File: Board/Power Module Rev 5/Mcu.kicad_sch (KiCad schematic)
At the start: 4 parts, among them J4 Conn_ARM_SWD_TagConnect_TC203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, J4 USB_C_Receptacle_USB2.0, U1 STM32G491CCUx, U6 MB85RS64

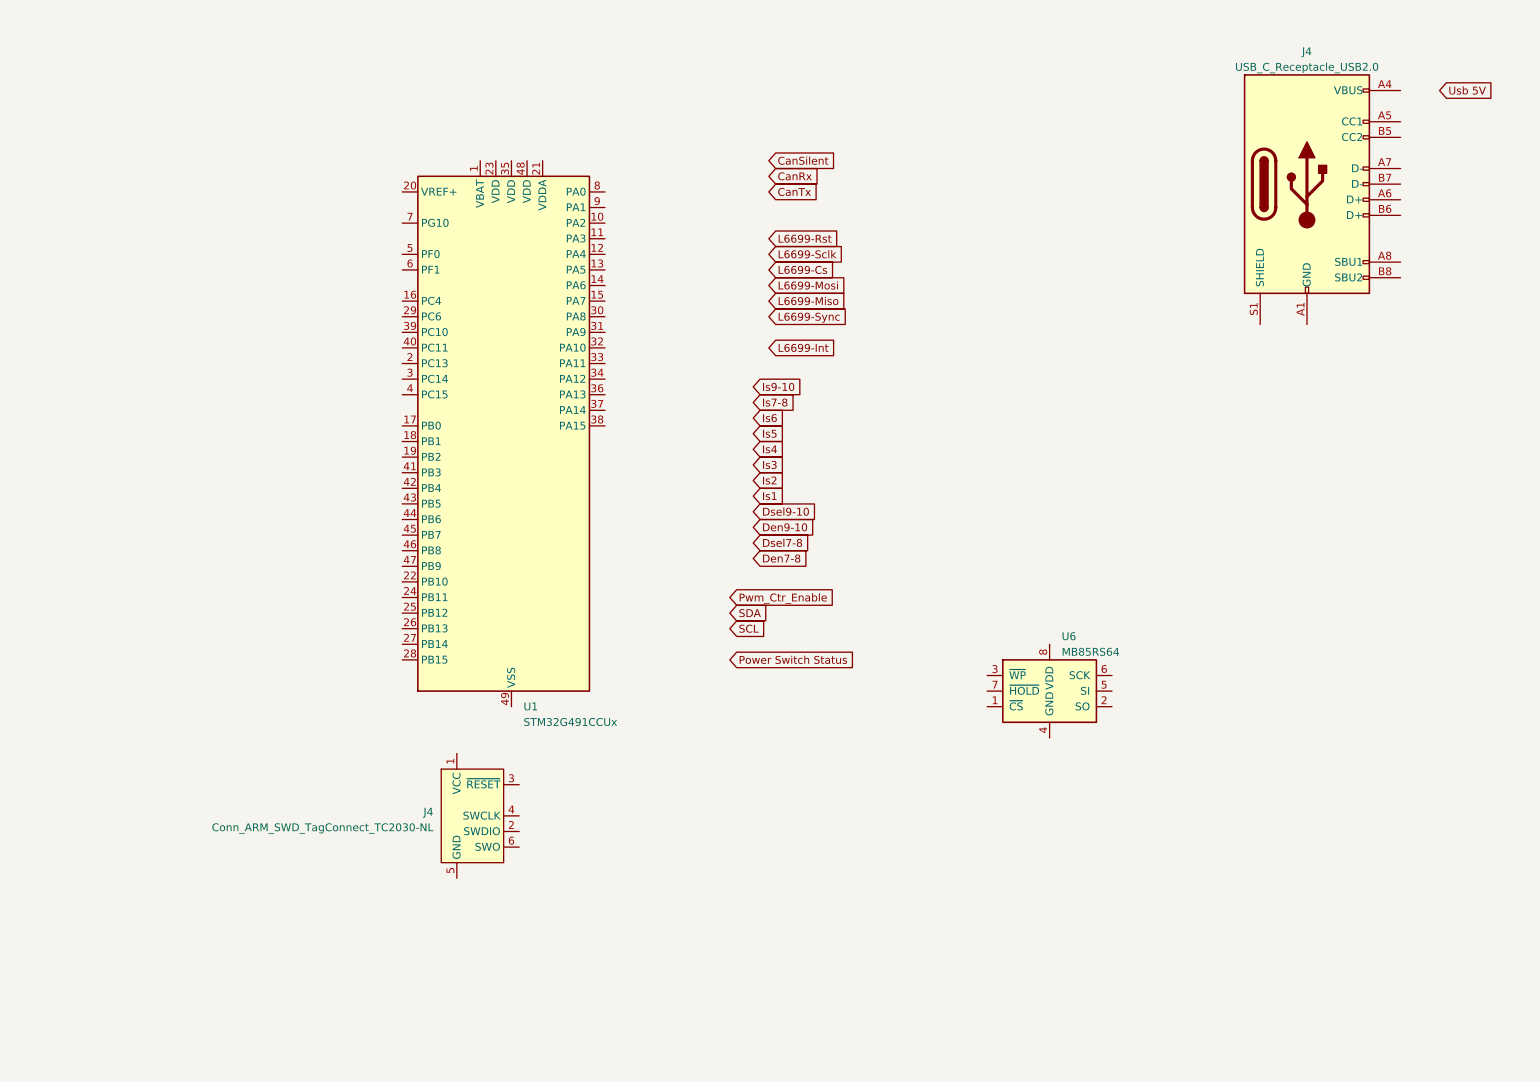
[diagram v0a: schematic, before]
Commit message: Board Update
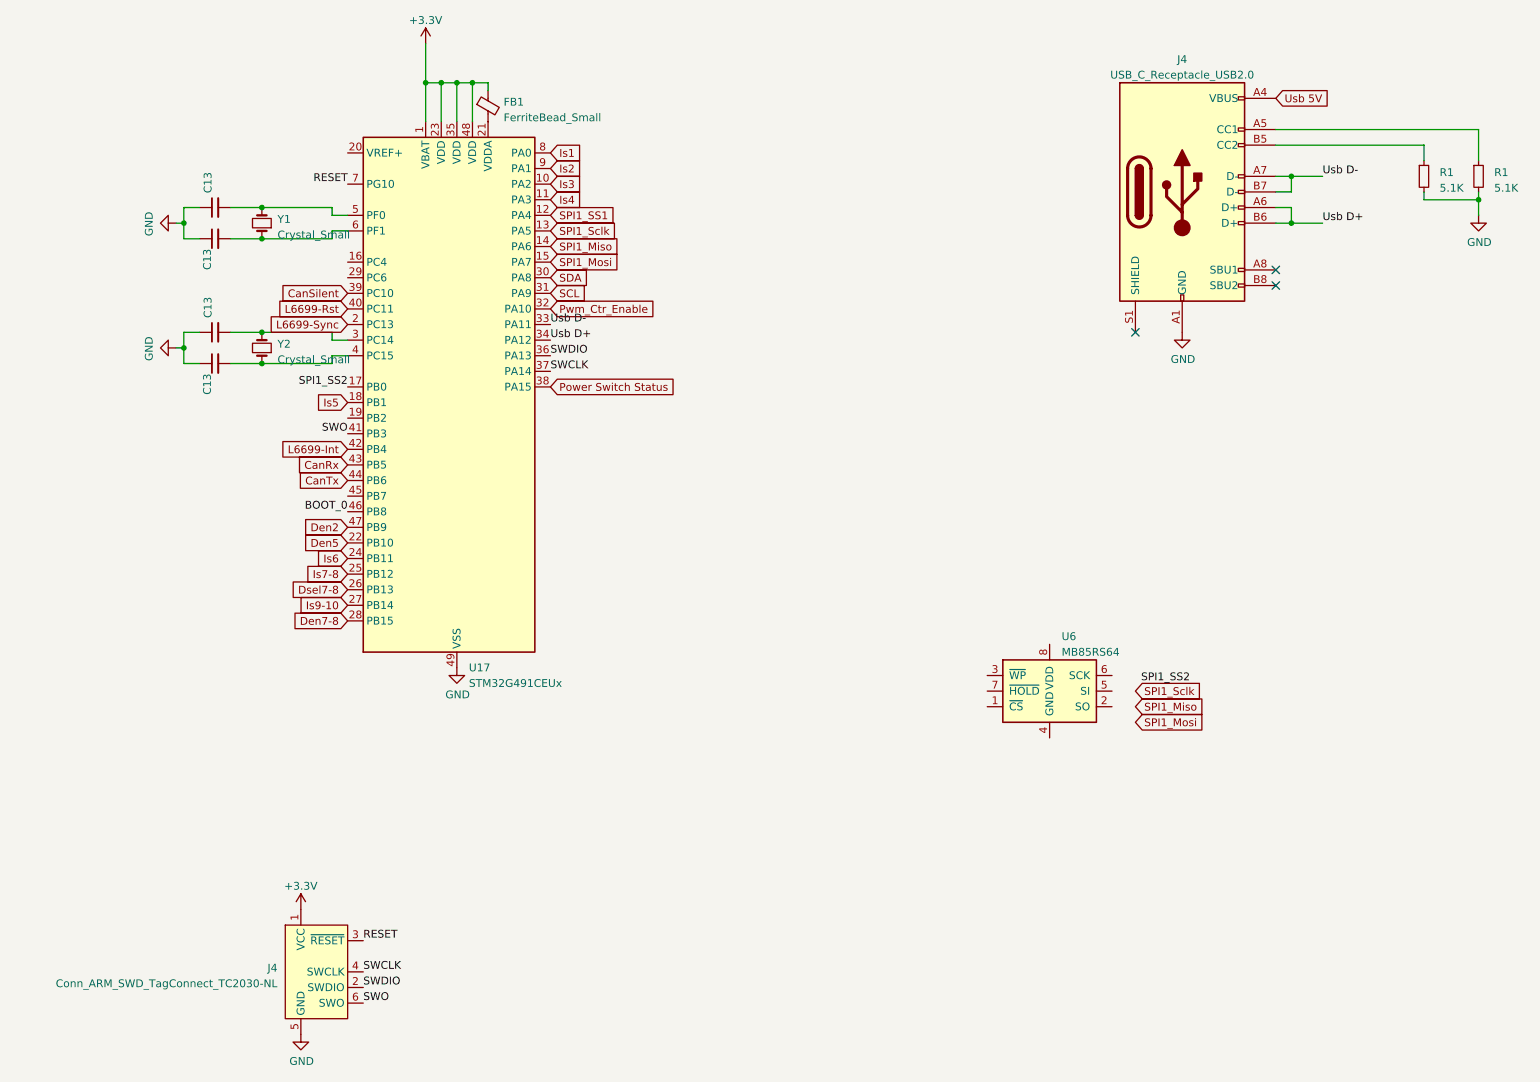
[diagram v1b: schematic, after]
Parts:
- removed U1: STM32G491CCUx, Package_DFN_QFN:QFN-48-1EP_7x7mm_P0.5mm_EP5.6x5.6mm, symbol MCU_ST_STM32G4:STM32G491CCUx
- added C13 (x4): ~, Capacitor_SMD:C_0603_1608Metric_Pad1.08x0.95mm_HandSolder, symbol Device:C_Small
- added FB1: FerriteBead_Small, Resistor_SMD:R_0603_1608Metric_Pad0.98x0.95mm_HandSolder, symbol Device:FerriteBead_Small
- added R1 (x2): 5.1K, Resistor_SMD:R_0603_1608Metric_Pad0.98x0.95mm_HandSolder, symbol Device:R_Small
- added U17: STM32G491CEUx, Package_DFN_QFN:QFN-48-1EP_7x7mm_P0.5mm_EP5.6x5.6mm, symbol MCU_ST_STM32G4:STM32G491CEUx
- added Y1, Y2: Crystal_Small, Crystal:Crystal_SMD_5032-2Pin_5.0x3.2mm, symbol Device:Crystal_Small
- J4: footprint (none) -> Connector_USB:USB_C_Receptacle_JAE_DX07S016JA1R1500
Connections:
- net CanRx: now also U17.43 (PB5)
- net CanSilent: now also U17.39 (PC10)
- net CanTx: now also U17.44 (PB6)
- net Den7-8: now also U17.28 (PB15)
- net Dsel7-8: now also U17.26 (PB13)
- net Is1: now also U17.8 (PA0)
- net Is2: now also U17.9 (PA1)
- net Is3: now also U17.10 (PA2)
- net Is4: now also U17.11 (PA3)
- net Is5: now also U17.18 (PB1)
- net Is6: now also U17.24 (PB11)
- net Is7-8: now also U17.25 (PB12)
- net Is9-10: now also U17.27 (PB14)
- net L6699-Int: now also U17.42 (PB4)
- net L6699-Rst: now also U17.40 (PC11)
- net L6699-Sync: now also U17.2 (PC13)
- net Power Switch Status: now also U17.38 (PA15)
- net Pwm_Ctr_Enable: now also U17.32 (PA10)
- net SCL: now also U17.31 (PA9)
- net SDA: now also U17.30 (PA8)
- net Usb 5V: now also J4.A4 (VBUS), J4.A9 (VBUS), J4.B4 (VBUS), J4.B9 (VBUS)
- net GND: now reaches J4.A1 (GND), J4.A12 (GND), J4.B1 (GND), J4.B12 (GND)
- net GND: now also J4.5 (GND), C13.1, C13.1, C13.1, C13.1, R1.2, R1.2, U17.49 (VSS)
- net at J4.A5 (CC1): now also R1.1
- net Usb D+: now reaches J4.A6 (D+)
- net Usb D+: now also J4.B6 (D+), U17.34 (PA12)
- net Usb D-: now reaches J4.A7 (D-)
- net Usb D-: now also J4.B7 (D-), U17.33 (PA11)
- net at J4.B5 (CC2): now also R1.1
- net +3.3V: now reaches J4.1 (VCC)
- net +3.3V: now also FB1.1, U17.1 (VBAT), U17.23 (VDD), U17.35 (VDD), U17.48 (VDD)
- net SWDIO: now reaches J4.2 (SWDIO)
- net SWDIO: now also U17.36 (PA13)
- net RESET: now reaches J4.3 (~{RESET})
- net RESET: now also U17.7 (PG10)
- net SWCLK: now reaches J4.4 (SWCLK)
- net SWCLK: now also U17.37 (PA14)
- net SWO: now reaches J4.6 (SWO)
- net SWO: now also U17.41 (PB3)
- new net: C13.2, U17.4 (PC15), Y2.1
- new net: C13.2, U17.3 (PC14), Y2.2
- new net: C13.2, U17.6 (PF1), Y1.1
- new net: FB1.2, U17.21 (VDDA)
- new net: C13.2, U17.5 (PF0), Y1.2
- new net BOOT_0: U17.46 (PB8)
- new net Den2: U17.47 (PB9)
- new net Den5: U17.22 (PB10)
- new net SPI1_Miso: U17.14 (PA6)
- new net SPI1_Mosi: U17.15 (PA7)
- new net SPI1_SS1: U17.12 (PA4)
- new net SPI1_SS2: U17.17 (PB0)
- new net SPI1_Sclk: U17.13 (PA5)
- no-connect marks 0 -> 3
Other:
- moved on the sheet: J4
